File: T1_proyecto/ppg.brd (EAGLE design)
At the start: 50 x 50 mm, 7 parts

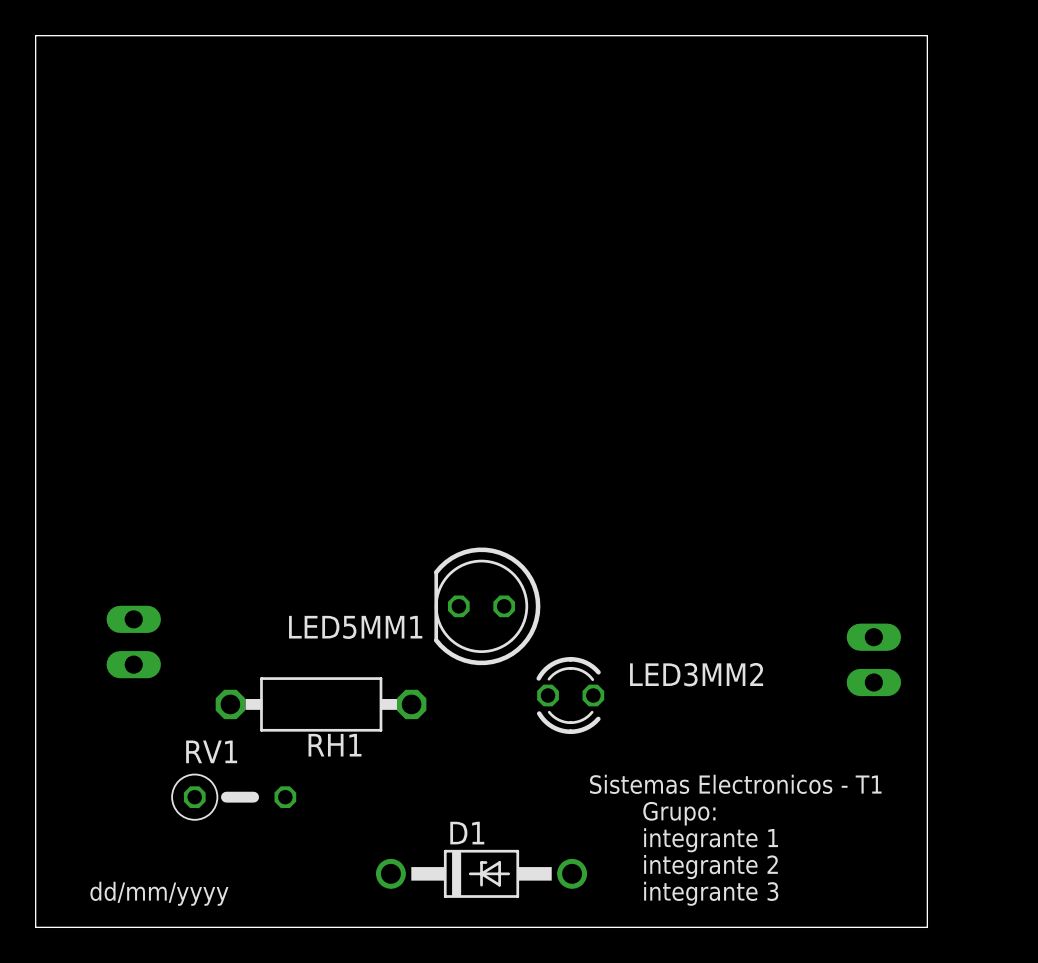
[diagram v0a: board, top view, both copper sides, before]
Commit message: update T1
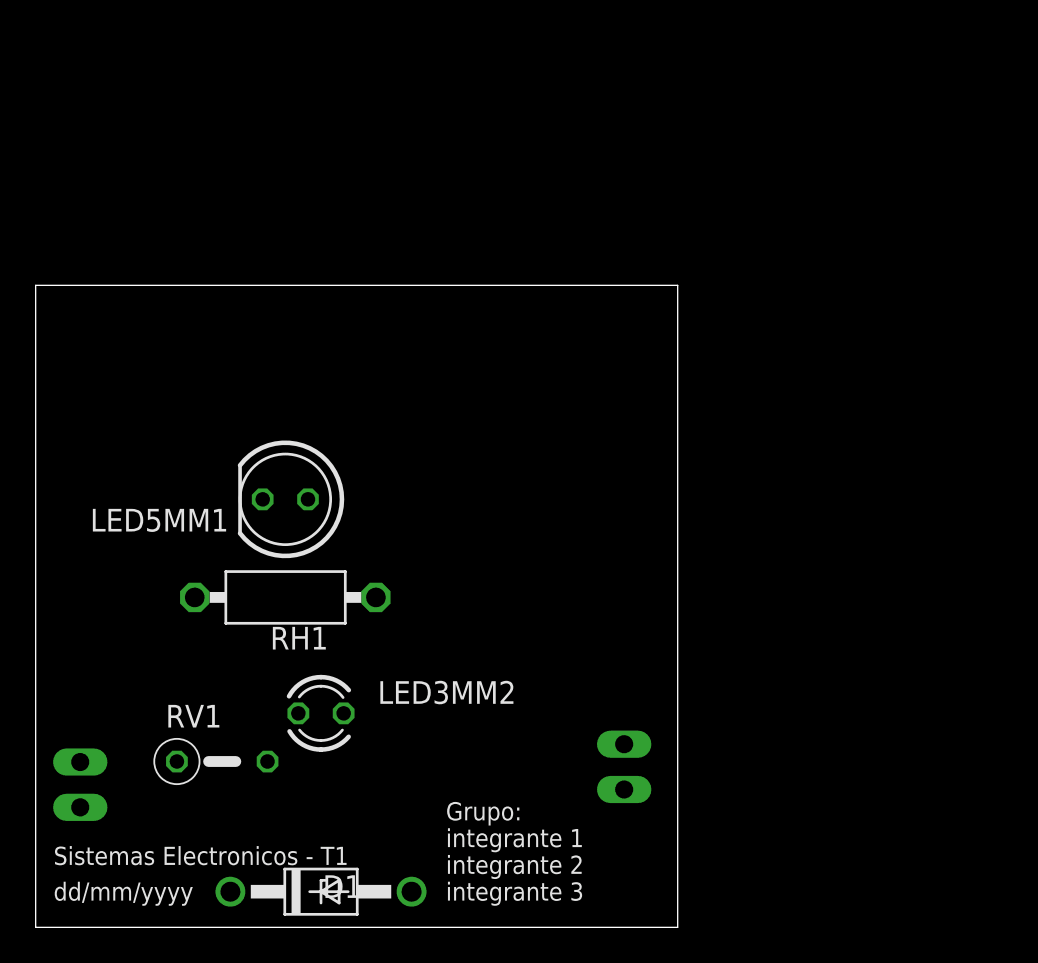
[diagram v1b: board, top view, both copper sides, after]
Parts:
- moved GND 15.2 mm to (33.0, 9.00)
- moved LED3MM2 14.0 mm to (16.0, 12.0)
- moved LED5MM1 12.5 mm to (14.0, 24.0)
- moved D1 9.06 mm to (16.0, 2.00)
- moved VI 8.54 mm to (2.50, 8.00)
- moved RH1 6.32 mm to (14.0, 18.5)
- moved RV1 2.24 mm to (10.5, 9.30)
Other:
- board size 50 x 50 mm -> 36 x 36 mm
